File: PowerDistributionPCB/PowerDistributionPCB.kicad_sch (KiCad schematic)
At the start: 40 parts, among them J1 USB3_A, Q1 AOD4185, U1 AP63203WU

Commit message: updated buck layout and edge cuts
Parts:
- C2, C3, C4: footprint Capacitor_SMD:C_0201_0603Metric_Pad0.64x0.40mm_HandSolder -> Capacitor_SMD:C_0603_1608Metric_Pad1.08x0.95mm_HandSolder
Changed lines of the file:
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@@
 			)
 		)
-		(property "Footprint" "Capacitor_SMD:C_0201_0603Metric_Pad0.64x0.40mm_HandSolder"
+		(property "Footprint" "Capacitor_SMD:C_0603_1608Metric_Pad1.08x0.95mm_HandSolder"
 			(at 164.7952 184.15 0)
 			(effects
@@
 			)
 		)
-		(property "Footprint" "Capacitor_SMD:C_0201_0603Metric_Pad0.64x0.40mm_HandSolder"
+		(property "Footprint" "Capacitor_SMD:C_0603_1608Metric_Pad1.08x0.95mm_HandSolder"
 			(at 140.97 173.0248 0)
 			(effects
@@
 			)
 		)
-		(property "Footprint" "Capacitor_SMD:C_0201_0603Metric_Pad0.64x0.40mm_HandSolder"
+		(property "Footprint" "Capacitor_SMD:C_0603_1608Metric_Pad1.08x0.95mm_HandSolder"
 			(at 154.6352 184.15 0)
 			(effects

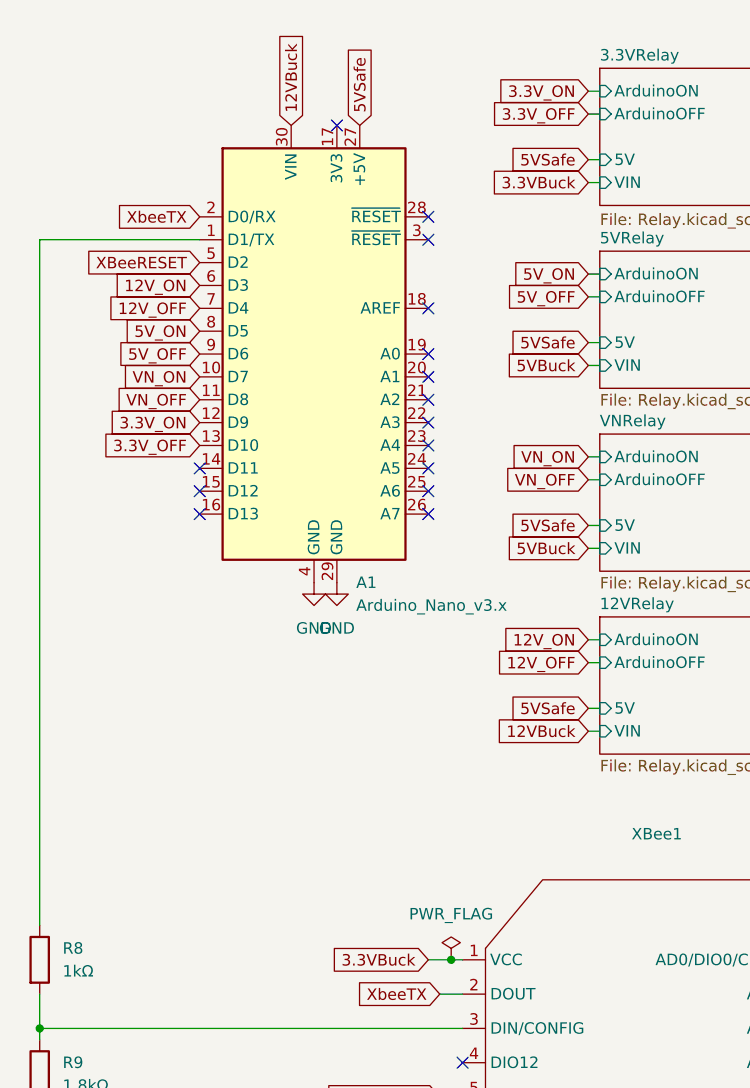
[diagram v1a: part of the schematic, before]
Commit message: fixing relay stuff
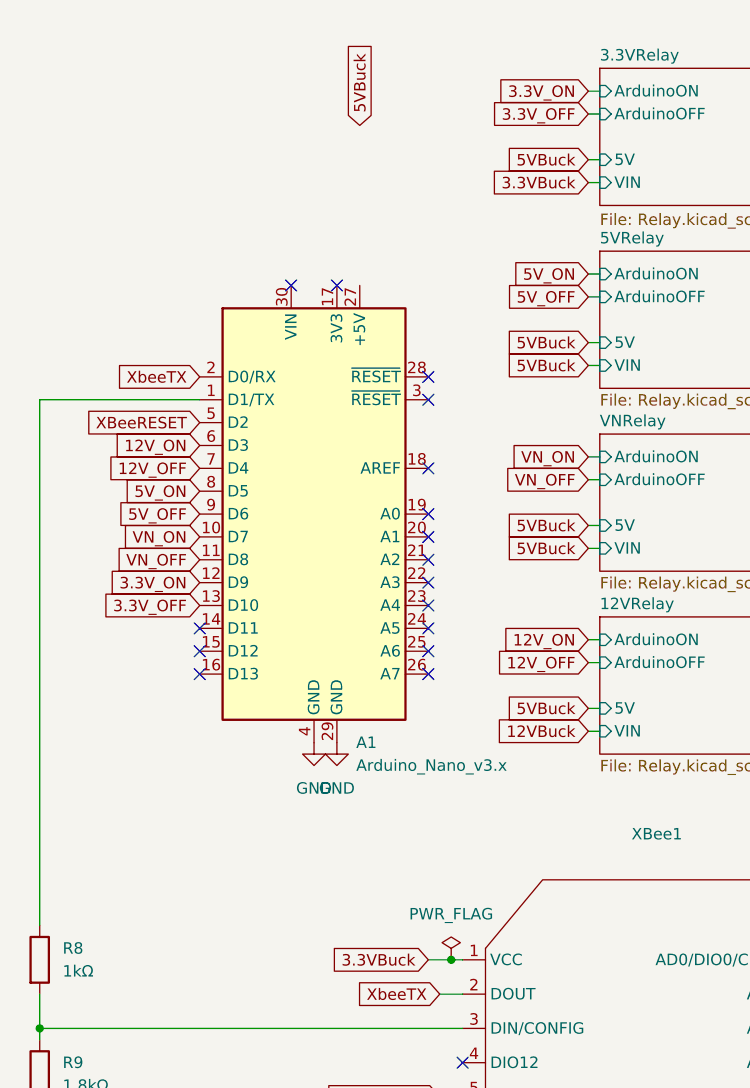
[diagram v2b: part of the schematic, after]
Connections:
- net 12VBuck: no longer A1.30 (VIN)
- net 5VSafe: no longer names the net of A1.27 (+5V)
- no-connect marks 42 -> 43
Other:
- moved on the sheet: A1
